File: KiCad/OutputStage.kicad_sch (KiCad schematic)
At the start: 42 parts, among them J2 Conn_Coaxial, Q1 BD135, Q2 BD136, U6 LM318H

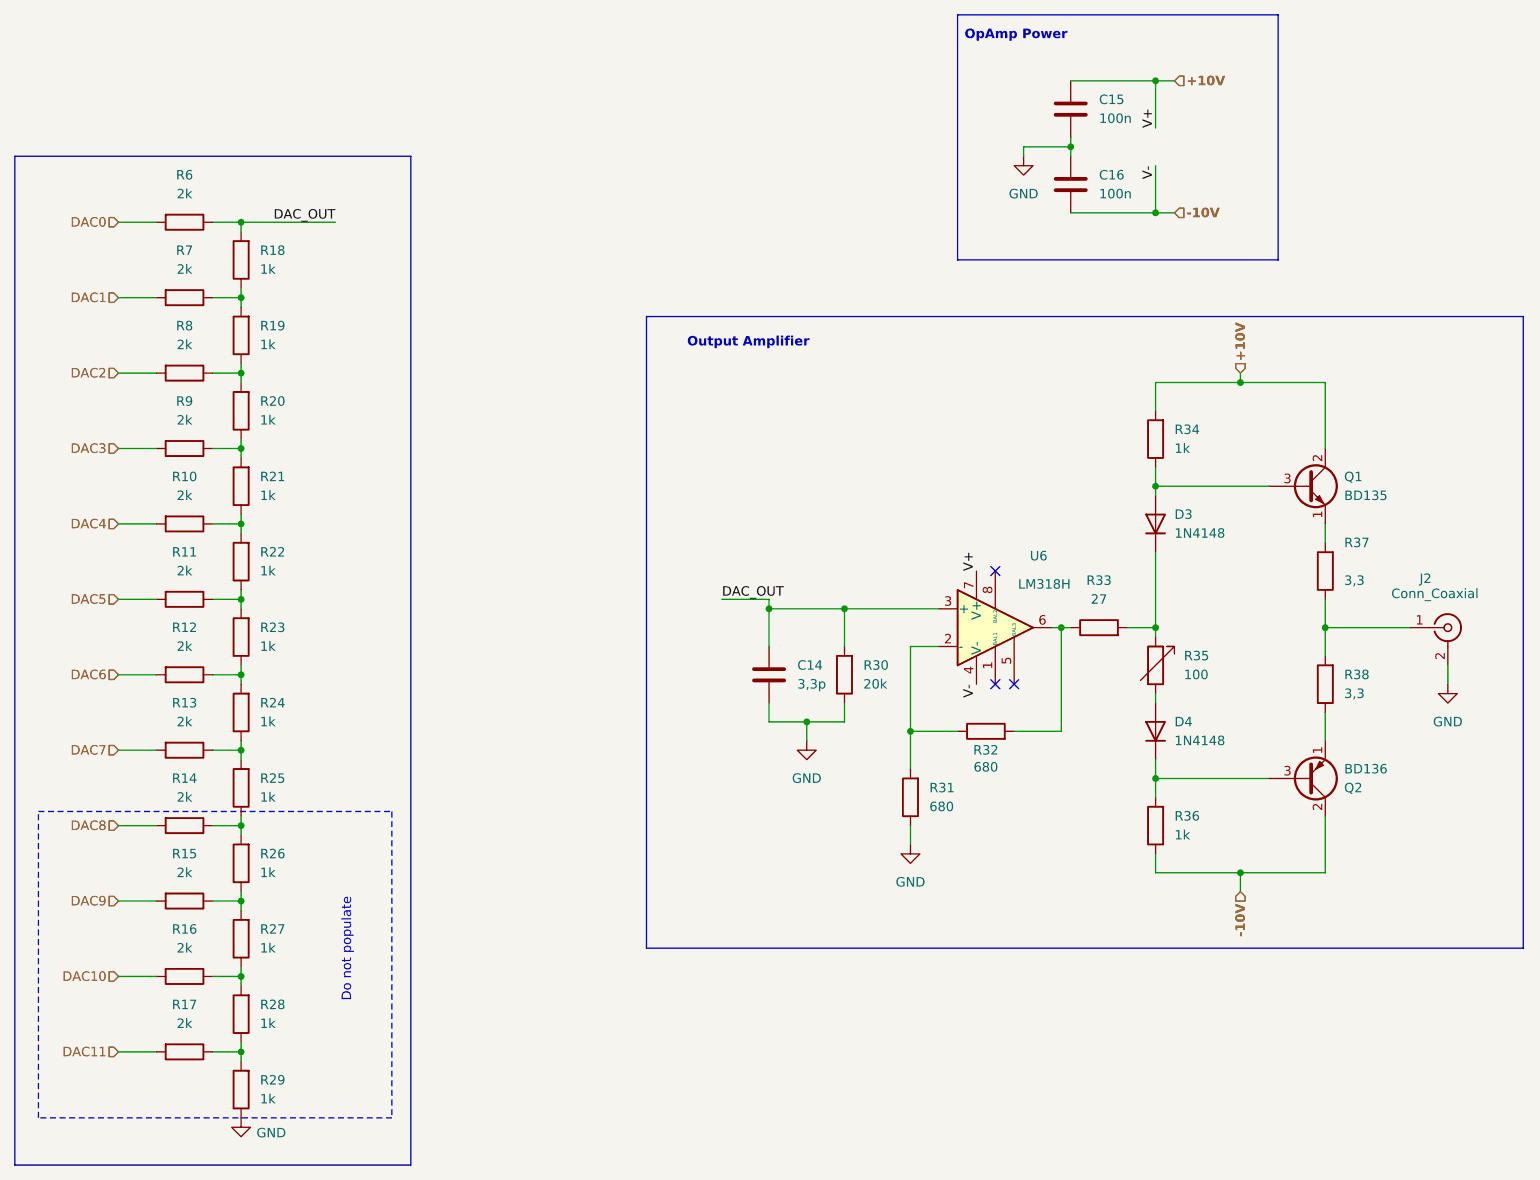
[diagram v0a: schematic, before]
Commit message: minor changes, testing
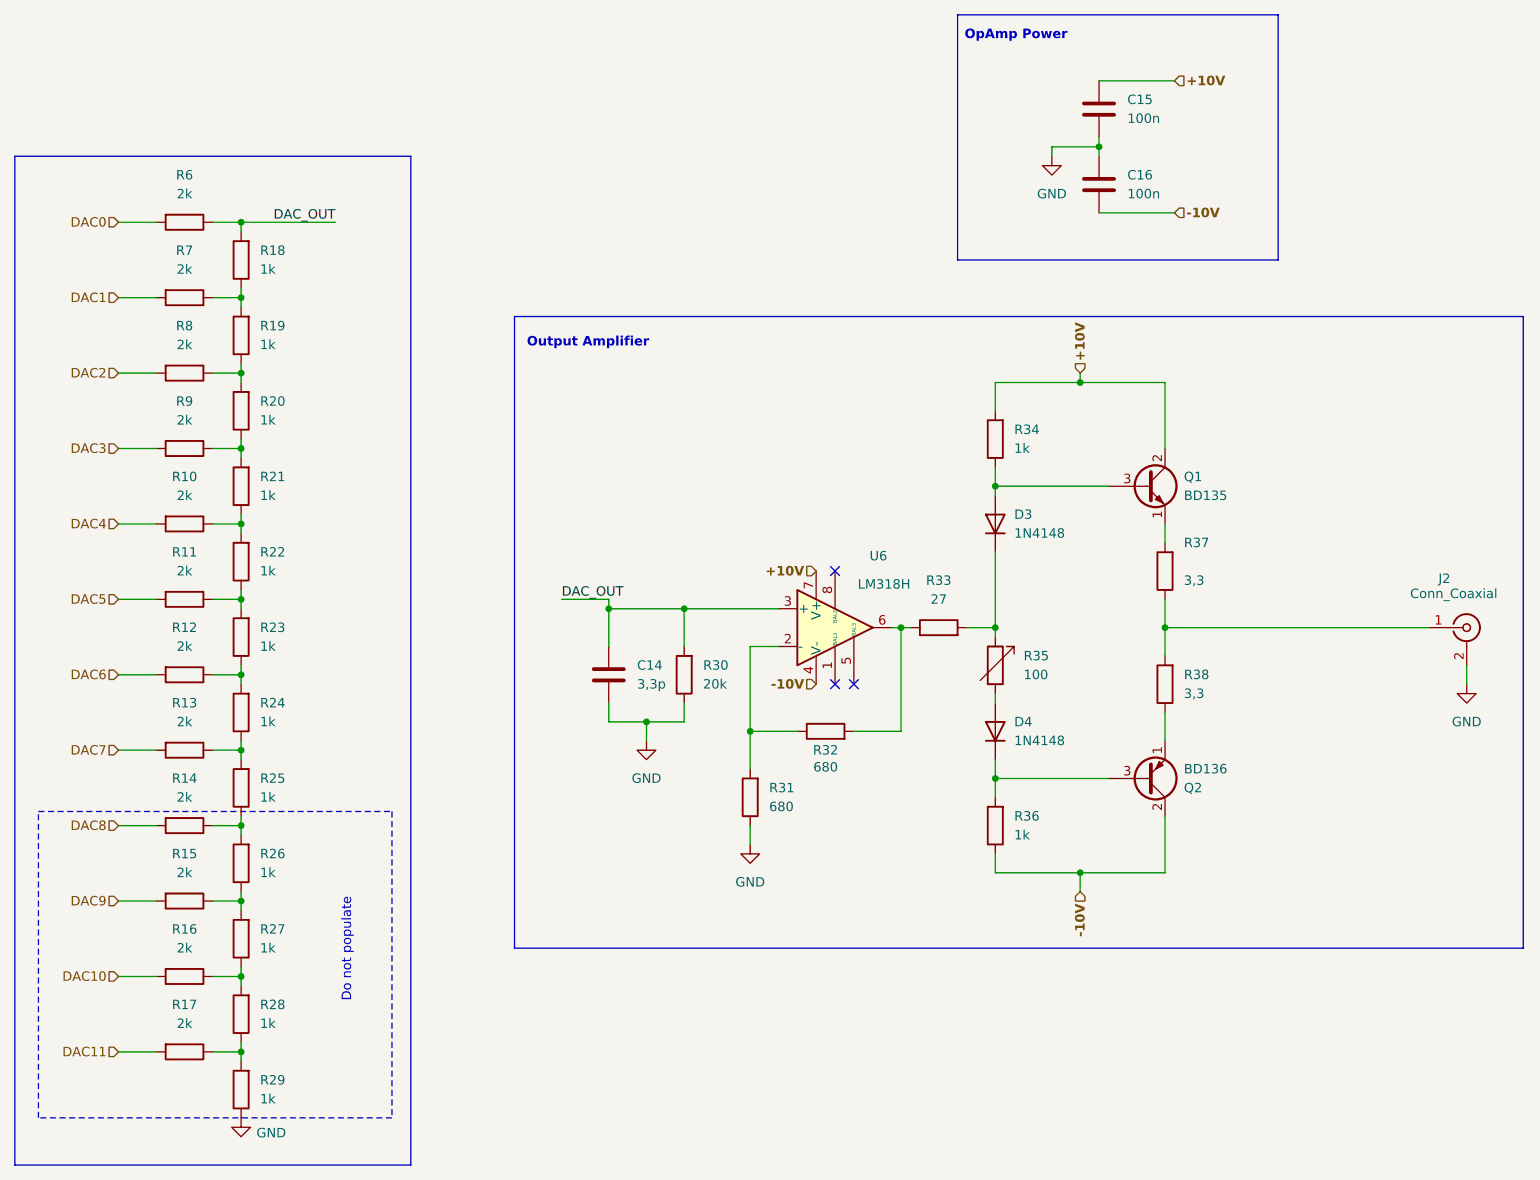
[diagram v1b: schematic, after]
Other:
- moved on the sheet: C14, C15, C16, D3, D4, J2, Q1, Q2, R30, R31, R32, R33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
